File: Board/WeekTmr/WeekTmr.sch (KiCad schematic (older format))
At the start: 24 parts, among them J11 TMR1.1, J12 TMR1.2, J21 TMR2.1, J22 TMR2.2, J3 Barrel_Jack_MountingPin, J4 DS3231, K1 FINDER-40.52, K2 FINDER-40.52, Q1 BC817, Q2 BC817, SW1 DOWN_BUT, SW2 UP_BUT, SW3 SELECT_BUT, U1 NHD-0420H1Z

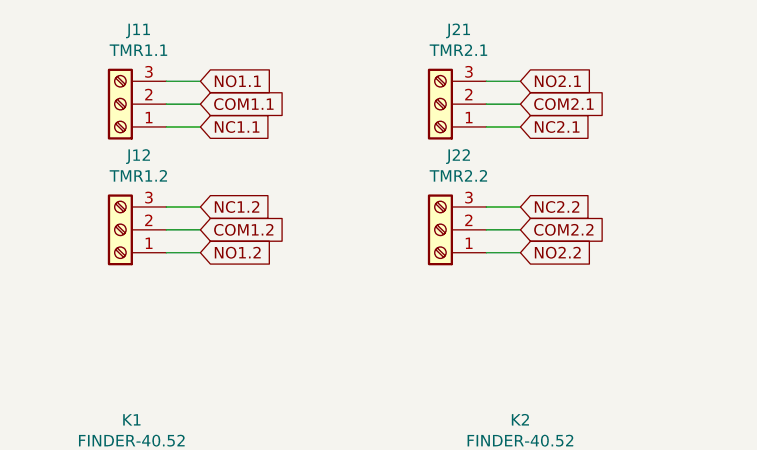
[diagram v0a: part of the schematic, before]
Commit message: board update
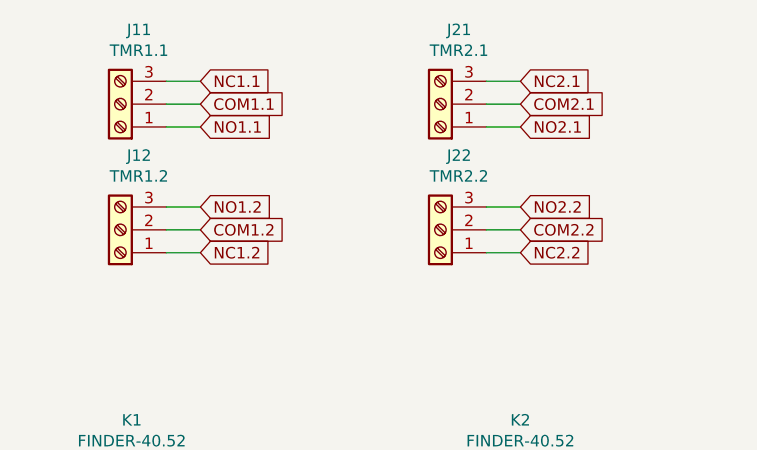
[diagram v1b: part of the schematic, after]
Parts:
- A1: footprint Module:Arduino_Nano -> KiCad_Library:Arduino_Nano_direct_Slot
- J11, J12, J21, J22: footprint TerminalBlock_Phoenix:TerminalBlock_Phoenix_MKDS-1,5-3-5.08_1x03_P5.08mm_Horizontal -> KiCad_Library:COMET_2EDGR-5.08-14-00AH
- R1, R2: footprint Resistor_SMD:R_0805_2012Metric_Pad1.15x1.40mm_HandSolder -> Resistor_THT:R_Axial_DIN0207_L6.3mm_D2.5mm_P15.24mm_Horizontal
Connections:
- net NC1.1: now also J11.3 (Pin_3); no longer J11.1 (Pin_1)
- net NC1.2: now also J12.1 (Pin_1); no longer J12.3 (Pin_3)
- net NC2.1: now also J21.3 (Pin_3); no longer J21.1 (Pin_1)
- net NC2.2: now also J22.1 (Pin_1); no longer J22.3 (Pin_3)
- net NO1.1: now also J11.1 (Pin_1); no longer J11.3 (Pin_3)
- net NO1.2: now also J12.3 (Pin_3); no longer J12.1 (Pin_1)
- net NO2.1: now also J21.1 (Pin_1); no longer J21.3 (Pin_3)
- net NO2.2: now also J22.3 (Pin_3); no longer J22.1 (Pin_1)
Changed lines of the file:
@@
 F 0 "A1" H 2400 3700 50  0000 C CNN
 F 1 "Arduino_Nano_v3.x" H 2700 3600 50  0000 C CNN
-F 2 "Module:Arduino_Nano" H 3350 2600 50  0001 C CIN
+F 2 "KiCad_Library:Arduino_Nano_direct_Slot" H 3350 2600 50  0001 C CIN
 F 3 "http://www.mouser.com/pdfdocs/Gravitech_Arduino_Nano3_0.pdf" H 3350 2600 50  0001 C CNN
 	1    3350 2600
@@
 F 0 "R1" V 7593 5050 50  0000 C CNN
 F 1 "R330" V 7684 5050 50  0000 C CNN
-F 2 "Resistor_SMD:R_0805_2012Metric_Pad1.15x1.40mm_HandSolder" V 7730 5050 50  0001 C CNN
+F 2 "Resistor_THT:R_Axial_DIN0207_L6.3mm_D2.5mm_P15.24mm_Horizontal" V 7730 5050 50  0001 C CNN
 F 3 "~" H 7800 5050 50  0001 C CNN
 	1    7800 5050
@@
 F 0 "R2" V 9293 5050 50  0000 C CNN
 F 1 "R330" V 9384 5050 50  0000 C CNN
-F 2 "Resistor_SMD:R_0805_2012Metric_Pad1.15x1.40mm_HandSolder" V 9430 5050 50  0001 C CNN
+F 2 "Resistor_THT:R_Axial_DIN0207_L6.3mm_D2.5mm_P15.24mm_Horizontal" V 9430 5050 50  0001 C CNN
 F 3 "~" H 9500 5050 50  0001 C CNN
 	1    9500 5050
@@
 F 0 "J21" H 9368 875 50  0000 C CNN
 F 1 "TMR2.1" H 9368 966 50  0000 C CNN
-F 2 "TerminalBlock_Phoenix:TerminalBlock_Phoenix_MKDS-1,5-3-5.08_1x03_P5.08mm_Horizontal" H 9450 1200 50  0001 C CNN
+F 2 "KiCad_Library:COMET_2EDGR-5.08-14-00AH" H 9450 1200 50  0001 C CNN
 F 3 "~" H 9450 1200 50  0001 C CNN
 	1    9450 1200
@@
 F 0 "J22" H 9368 1425 50  0000 C CNN
 F 1 "TMR2.2" H 9368 1516 50  0000 C CNN
-F 2 "TerminalBlock_Phoenix:TerminalBlock_Phoenix_MKDS-1,5-3-5.08_1x03_P5.08mm_Horizontal" H 9450 1750 50  0001 C CNN
+F 2 "KiCad_Library:COMET_2EDGR-5.08-14-00AH" H 9450 1750 50  0001 C CNN
 F 3 "~" H 9450 1750 50  0001 C CNN
 	1    9450 1750
@@
 F 0 "J11" H 7968 875 50  0000 C CNN
 F 1 "TMR1.1" H 7968 966 50  0000 C CNN
-F 2 "TerminalBlock_Phoenix:TerminalBlock_Phoenix_MKDS-1,5-3-5.08_1x03_P5.08mm_Horizontal" H 8050 1200 50  0001 C CNN
+F 2 "KiCad_Library:COMET_2EDGR-5.08-14-00AH" H 8050 1200 50  0001 C CNN
 F 3 "~" H 8050 1200 50  0001 C CNN
 	1    8050 1200
@@
 F 0 "J12" H 7968 1425 50  0000 C CNN
 F 1 "TMR1.2" H 7968 1516 50  0000 C CNN
-F 2 "TerminalBlock_Phoenix:TerminalBlock_Phoenix_MKDS-1,5-3-5.08_1x03_P5.08mm_Horizontal" H 8050 1750 50  0001 C CNN
+F 2 "KiCad_Library:COMET_2EDGR-5.08-14-00AH" H 8050 1750 50  0001 C CNN
 F 3 "~" H 8050 1750 50  0001 C CNN
 	1    8050 1750
@@
 Text GLabel 9800 1750 2    50   Input ~ 0
 COM2.2
+Text GLabel 8400 1300 2    50   Input ~ 0
+NO1.1
 Text GLabel 8400 1100 2    50   Input ~ 0
-NO1.1
-Text GLabel 8400 1300 2    50   Input ~ 0
 NC1.1
 Wire Wire Line
-	8250 1300 8400 1300
-Wire Wire Line
 	8250 1200 8400 1200
-Wire Wire Line
-	8250 1100 8400 1100
+Text GLabel 8400 1650 2    50   Input ~ 0
+NO1.2
 Text GLabel 8400 1850 2    50   Input ~ 0
-NO1.2
-Text GLabel 8400 1650 2    50   Input ~ 0
 NC1.2
+Text GLabel 9800 1300 2    50   Input ~ 0
+NO2.1
 Text GLabel 9800 1100 2    50   Input ~ 0
-NO2.1
-Text GLabel 9800 1300 2    50   Input ~ 0
 NC2.1
 Wire Wire Line
-	9650 1100 9800 1100
-Wire Wire Line
 	9650 1200 9800 1200
-Wire Wire Line
-	9650 1300 9800 1300
+Text GLabel 9800 1650 2    50   Input ~ 0
+NO2.2
 Text GLabel 9800 1850 2    50   Input ~ 0
-NO2.2
-Text GLabel 9800 1650 2    50   Input ~ 0
 NC2.2
 Wire Wire Line
-	9650 1650 9800 1650
-Wire Wire Line
 	9650 1750 9800 1750
 Wire Wire Line
-	9650 1850 9800 1850
-Wire Wire Line
-	8250 1650 8400 1650
-Wire Wire Line
 	8250 1750 8400 1750
-Wire Wire Line
-	8250 1850 8400 1850
 $Comp
 L Diode:1N5819 D2
@@
 Wire Wire Line
 	10100 4250 10100 4600
+Wire Wire Line
+	8250 1100 8400 1100
+Wire Wire Line
+	8250 1300 8400 1300
+Wire Wire Line
+	8250 1650 8400 1650
+Wire Wire Line
+	8250 1850 8400 1850
+Wire Wire Line
+	9650 1100 9800 1100
+Wire Wire Line
+	9650 1300 9800 1300
+Wire Wire Line
+	9650 1650 9800 1650
+Wire Wire Line
+	9650 1850 9800 1850
 $EndSCHEMATC
